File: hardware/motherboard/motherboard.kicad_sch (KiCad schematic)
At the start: 82 parts, among them J1 IMU Connector, J2 JST-VH, J3 JST-VH, J4 JST-PH, J5 USB C 2.0, Q1 TSM7P06CP_ROG, Q2 TSM7P06CP_ROG, SW1 A, SW10 Right, SW11 Left, SW12 Up, SW13 Reset, SW2 B, SW3 X, SW4 Y, SW5 LB, SW6 RB, SW7 Start, SW8 Select, SW9 Down, U1 ESP32-S3-WROOM-1, U2 MCP73831-2-OT, U3 TPS75533KTTRG3, U4 TLV75709PDBV, U5 COM-09032

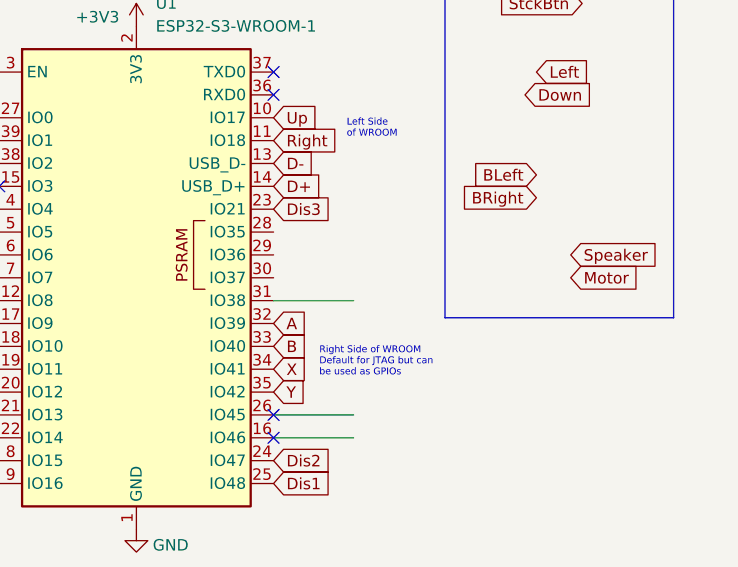
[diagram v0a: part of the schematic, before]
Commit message: Right Side Controls Routing
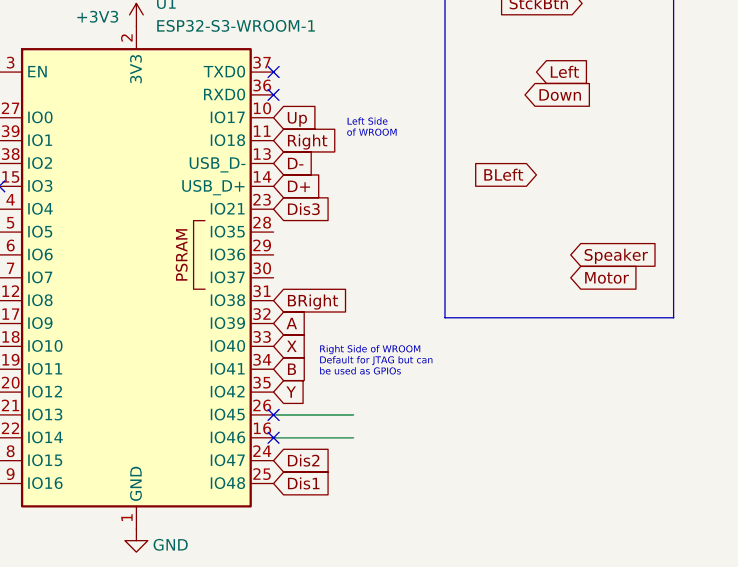
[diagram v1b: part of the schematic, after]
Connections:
- net B: now also U1.34 (IO41); no longer U1.33 (IO40)
- net BRight: now also U1.31 (IO38)
- net X: now also U1.33 (IO40); no longer U1.34 (IO41)
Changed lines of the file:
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@@
-	(wire
-		(pts
-			(xy 237.49 55.88) (xy 246.38 55.88)
-		)
-		(stroke
-			(width 0)
-			(type default)
-		)
-	)
 	(wire
 		(pts
@@
 	(global_label "BRight"
 		(shape input)
-		(at 266.7 44.45 180)
-		(fields_autoplaced yes)
-		(effects
-			(font
-				(size 1.27 1.27)
-			)
-			(justify right)
-		)
-		(property "Intersheetrefs" "${INTERSHEET_REFS}"
-			(at 257.5463 44.45 0)
-			(effects
-				(font
-					(size 1.27 1.27)
-				)
-				(justify right)
+		(at 237.49 55.88 0)
+		(fields_autoplaced yes)
+		(effects
+			(font
+				(size 1.27 1.27)
+			)
+			(justify left)
+		)
+		(property "Intersheetrefs" "${INTERSHEET_REFS}"
+			(at 246.6437 55.88 0)
+			(effects
+				(font
+					(size 1.27 1.27)
+				)
+				(justify left)
 				(hide yes)
 			)
@@
 	(global_label "B"
 		(shape input)
+		(at 237.49 63.5 0)
+		(fields_autoplaced yes)
+		(effects
+			(font
+				(size 1.27 1.27)
+			)
+			(justify left)
+		)
+		(property "Intersheetrefs" "${INTERSHEET_REFS}"
+			(at 241.7452 63.5 0)
+			(effects
+				(font
+					(size 1.27 1.27)
+				)
+				(justify left)
+				(hide yes)
+			)
+		)
+	)
+	(global_label "ACC1"
+		(shape input)
+		(at 147.32 133.35 0)
+		(fields_autoplaced yes)
+		(effects
+			(font
+				(size 1.27 1.27)
+			)
+			(justify left)
+		)
+		(property "Intersheetrefs" "${INTERSHEET_REFS}"
+			(at 155.1433 133.35 0)
+			(effects
+				(font
+					(size 1.27 1.27)
+				)
+				(justify left)
+				(hide yes)
+			)
+		)
+	)
+	(global_label "VPeripheral"
+		(shape input)
+		(at 226.06 143.51 180)
+		(fields_autoplaced yes)
+		(effects
+			(font
+				(size 1.27 1.27)
+			)
+			(justify right)
+		)
+		(property "Intersheetrefs" "${INTERSHEET_REFS}"
+			(at 212.2496 143.51 0)
+			(effects
+				(font
+					(size 1.27 1.27)
+				)
+				(justify right)
+				(hide yes)
+			)
+		)
+	)
+	(global_label "D+"
+		(shape input)
+		(at 66.04 163.83 0)
+		(fields_autoplaced yes)
+		(effects
+			(font
+				(size 1.27 1.27)
+			)
+			(justify left)
+		)
+		(property "Intersheetrefs" "${INTERSHEET_REFS}"
+			(at 71.8676 163.83 0)
+			(effects
+				(font
+					(size 1.27 1.27)
+				)
+				(justify left)
+				(hide yes)
+			)
+		)
+	)
+	(global_label "X"
+		(shape input)
 		(at 237.49 60.96 0)
 		(fields_autoplaced yes)
@@
 		)
 		(property "Intersheetrefs" "${INTERSHEET_REFS}"
-			(at 241.7452 60.96 0)
-			(effects
-				(font
-					(size 1.27 1.27)
-				)
-				(justify left)
-				(hide yes)
-			)
-		)
-	)
-	(global_label "ACC1"
-		(shape input)
-		(at 147.32 133.35 0)
-		(fields_autoplaced yes)
-		(effects
-			(font
-				(size 1.27 1.27)
-			)
-			(justify left)
-		)
-		(property "Intersheetrefs" "${INTERSHEET_REFS}"
-			(at 155.1433 133.35 0)
-			(effects
-				(font
-					(size 1.27 1.27)
-				)
-				(justify left)
-				(hide yes)
-			)
-		)
-	)
-	(global_label "VPeripheral"
-		(shape input)
-		(at 226.06 143.51 180)
-		(fields_autoplaced yes)
-		(effects
-			(font
-				(size 1.27 1.27)
-			)
-			(justify right)
-		)
-		(property "Intersheetrefs" "${INTERSHEET_REFS}"
-			(at 212.2496 143.51 0)
-			(effects
-				(font
-					(size 1.27 1.27)
-				)
-				(justify right)
-				(hide yes)
-			)
-		)
-	)
-	(global_label "D+"
-		(shape input)
-		(at 66.04 163.83 0)
-		(fields_autoplaced yes)
-		(effects
-			(font
-				(size 1.27 1.27)
-			)
-			(justify left)
-		)
-		(property "Intersheetrefs" "${INTERSHEET_REFS}"
-			(at 71.8676 163.83 0)
-			(effects
-				(font
-					(size 1.27 1.27)
-				)
-				(justify left)
-				(hide yes)
-			)
-		)
-	)
-	(global_label "X"
-		(shape input)
-		(at 237.49 63.5 0)
-		(fields_autoplaced yes)
-		(effects
-			(font
-				(size 1.27 1.27)
-			)
-			(justify left)
-		)
-		(property "Intersheetrefs" "${INTERSHEET_REFS}"
-			(at 241.6847 63.5 0)
-			(effects
-				(font
+			(at 241.6847 60.96 0)
+			(effects
+				(font
